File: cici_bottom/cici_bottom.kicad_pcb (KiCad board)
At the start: 2 copper layers, 88.4 x 132.8 mm, 8 parts

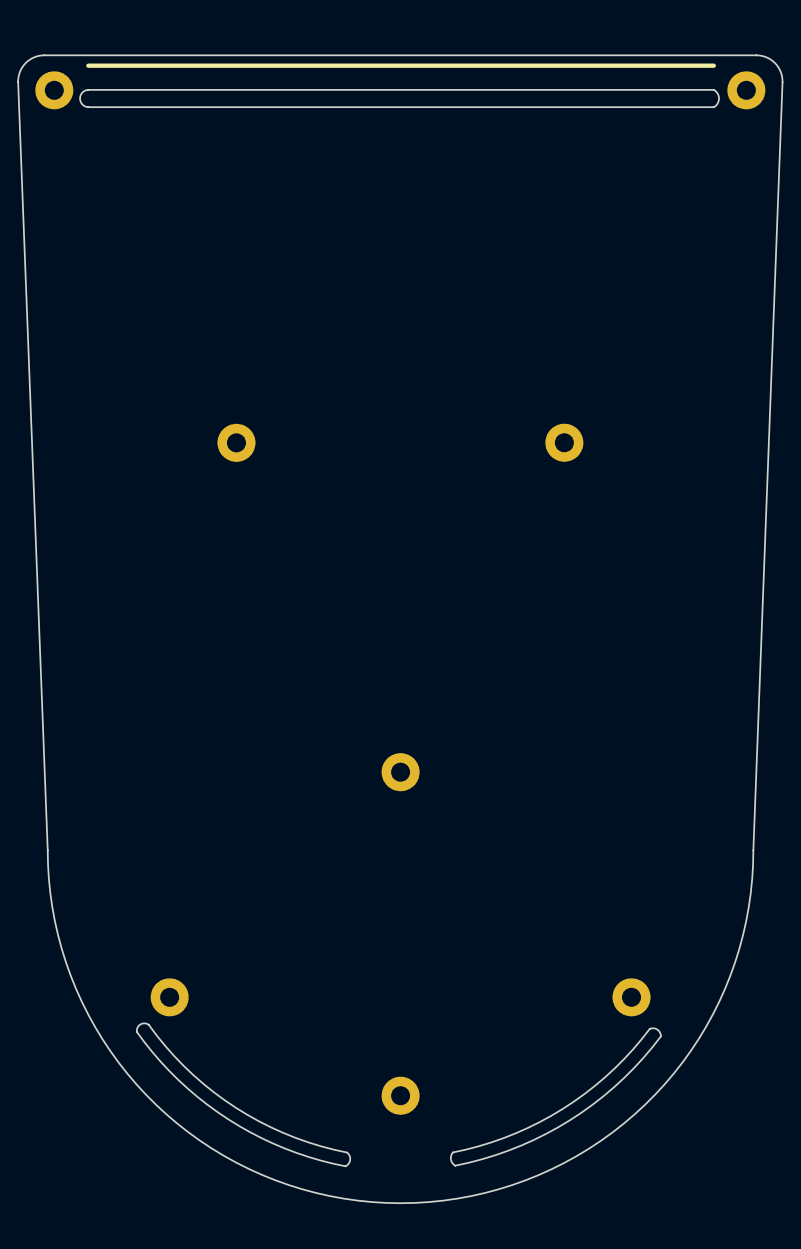
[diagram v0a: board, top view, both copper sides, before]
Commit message: prima versione conclusa. inizio seconda
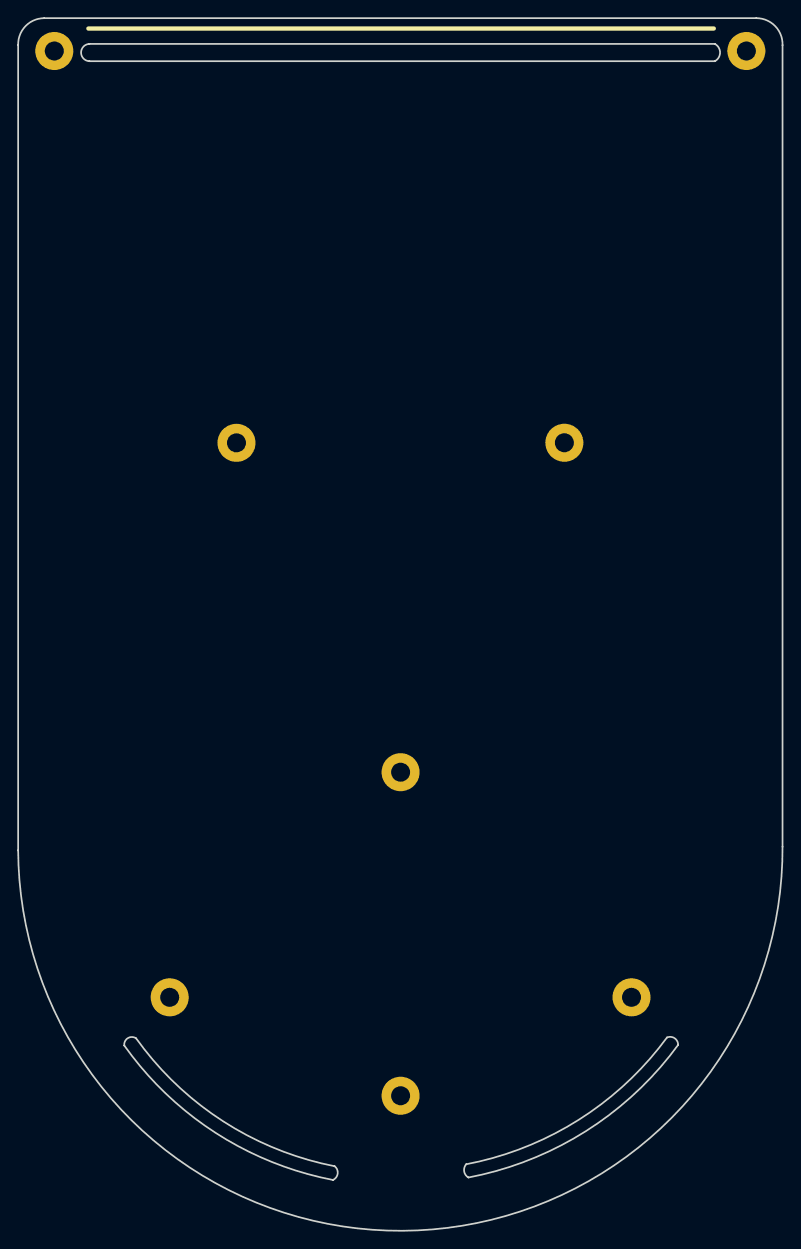
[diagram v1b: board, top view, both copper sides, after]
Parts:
- moved REF** 4.55 mm to (54.1, 25.5)
- moved REF** 4.55 mm to (134.1, 25.5)
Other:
- board size 88.4 x 132.8 mm -> 88.4 x 140.3 mm
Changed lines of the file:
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@@
   )
   (module MountingHole:MountingHole_2.2mm_M2_Pad (layer F.Cu)
-    (at 54.06 30.05)
+    (at 54.06 25.5)
     (descr "Mounting Hole 2.2mm, M2")
     (tags "mounting hole 2.2mm m2")
@@
   )
   (module MountingHole:MountingHole_2.2mm_M2_Pad (layer F.Cu)
-    (at 134.14 30.05)
+    (at 134.14 25.5)
     (descr "Mounting Hole 2.2mm, M2")
     (tags "mounting hole 2.2mm m2")
@@
     (pad 1 thru_hole circle (at 0 0) (size 4.4 4.4) (drill 2.2) (layers *.Cu *.Mask))
   )
-  (gr_line (start 58 27.2) (end 130.375 27.2) (layer F.SilkS) (width 0.5))
-  (gr_arc (start 123.33 139.5) (end 124.246762 139.525368) (angle -115.3397962) (layer Edge.Cuts) (width 0.2))
-  (gr_arc (start 100.95 153.61) (end 100.191271 152.951118) (angle -101.2542279) (layer Edge.Cuts) (width 0.2))
-  (gr_arc (start 64.48 138.89) (end 64.98 138.17) (angle -131.9838884) (layer Edge.Cuts) (width 0.2))
-  (gr_arc (start 87.37 153.7) (end 87.750789 154.553857) (angle -117.7344543) (layer Edge.Cuts) (width 0.2))
-  (gr_arc (start 92.926271 116.091118) (end 100.191271 152.951118) (angle -41.92680981) (layer Edge.Cuts) (width 0.2))
-  (gr_arc (start 95.075 116.675) (end 64.98 138.17) (angle -43.3547479) (layer Edge.Cuts) (width 0.2))
-  (gr_arc (start 92.925 116.1) (end 100.451863 154.482728) (angle -42.11246634) (layer Edge.Cuts) (width 0.2))
-  (gr_arc (start 95.075 116.675) (end 63.61 139) (angle -43.7) (layer Edge.Cuts) (width 0.2))
-  (gr_arc (start 58.04 31) (end 58 32) (angle 175.4) (layer Edge.Cuts) (width 0.2))
-  (gr_arc (start 129.84 31) (end 130.375 32) (angle -123.7064376) (layer Edge.Cuts) (width 0.2))
-  (gr_line (start 58 32) (end 130.375 32) (layer Edge.Cuts) (width 0.2))
-  (gr_line (start 58 30) (end 130.375 30) (layer Edge.Cuts) (width 0.2))
-  (gr_text CICI (at 94.125 153.3) (layer B.SilkS)
-    (effects (font (size 4 4) (thickness 0.5)) (justify mirror))
+  (gr_arc (start 85.92 155.28) (end 86.300789 156.133857) (angle -117.7344543) (layer Edge.Cuts) (width 0.2))
+  (gr_arc (start 63.03 140.47) (end 63.53 139.75) (angle -131.9838884) (layer Edge.Cuts) (width 0.2))
+  (gr_arc (start 93.625 118.255) (end 63.53 139.75) (angle -43.3547479) (layer Edge.Cuts) (width 0.2))
+  (gr_arc (start 93.625 118.255) (end 62.16 140.58) (angle -43.7) (layer Edge.Cuts) (width 0.2))
+  (gr_line (start 58 22.9) (end 130.375 22.9) (layer F.SilkS) (width 0.5))
+  (gr_arc (start 125.32217 140.491405) (end 126.238932 140.516773) (angle -115.3397962) (layer Edge.Cuts) (width 0.2))
+  (gr_arc (start 102.478137 154.977272) (end 101.719408 154.31839) (angle -101.2542279) (layer Edge.Cuts) (width 0.2))
+  (gr_arc (start 94.666271 117.411118) (end 101.719408 154.31839) (angle -42.88924805) (layer Edge.Cuts) (width 0.2))
+  (gr_arc (start 94.665 117.42) (end 101.98 155.85) (angle -43.03690352) (layer Edge.Cuts) (width 0.2))
+  (gr_arc (start 58.16 25.68) (end 58.12 26.68) (angle 175.4) (layer Edge.Cuts) (width 0.2))
+  (gr_arc (start 129.96 25.68) (end 130.495 26.68) (angle -123.7064376) (layer Edge.Cuts) (width 0.2))
+  (gr_line (start 58.12 26.68) (end 130.495 26.68) (layer Edge.Cuts) (width 0.2))
+  (gr_line (start 58.12 24.68) (end 130.495 24.68) (layer Edge.Cuts) (width 0.2))
+  (gr_text CICI (at 94.13 155.5) (layer B.SilkS)
+    (effects (font (size 3 4) (thickness 0.5)) (justify mirror))
   )
-  (gr_text -zanni- (at 94.125 149.7) (layer B.SilkS)
+  (gr_text -zanni- (at 94.13 152) (layer B.SilkS)
     (effects (font (size 1.5 1.5) (thickness 0.3)) (justify mirror))
   )
-  (gr_arc (start 92.925 116.1) (end 100.3 155.55) (angle -43.4) (layer B.SilkS) (width 0.5))
-  (gr_arc (start 95.075 116.675) (end 62.9 139.75) (angle -44.1) (layer B.SilkS) (width 0.5))
-  (gr_arc (start 94.15 117.85) (end 54.525 118.4) (angle -179.2) (layer B.SilkS) (width 0.5))
-  (gr_line (start 54.525 118.4) (end 51.100929 34) (layer B.SilkS) (width 0.5))
-  (gr_line (start 137.153817 34) (end 133.778817 117.853305) (layer B.SilkS) (width 0.5))
-  (gr_line (start 58 27.2) (end 130.375 27.2) (layer B.SilkS) (width 0.5))
-  (gr_arc (start 135.3 29.025) (end 138.325 29.125) (angle -91.9) (layer Edge.Cuts) (width 0.2))
-  (gr_line (start 138.325 29.125) (end 134.95 118) (layer Edge.Cuts) (width 0.2))
-  (gr_arc (start 94.125 118) (end 53.3 118) (angle -180) (layer Edge.Cuts) (width 0.2))
-  (gr_line (start 53.3 118) (end 49.875929 29.099977) (layer Edge.Cuts) (width 0.2))
-  (gr_arc (start 52.9 29.025) (end 52.9 26) (angle -91.4) (layer Edge.Cuts) (width 0.2))
-  (gr_line (start 52.9 26) (end 135.3 26) (layer Edge.Cuts) (width 0.2))
+  (gr_arc (start 94.1227 117.42) (end 100.53 158.33) (angle -43.4) (layer B.SilkS) (width 0.5))
+  (gr_arc (start 94.1227 117.42) (end 61.73 143.22) (angle -42.90512361) (layer B.SilkS) (width 0.5))
+  (gr_arc (start 94.1227 117.42) (end 51.100929 118.4) (angle -179.2) (layer B.SilkS) (width 0.5))
+  (gr_line (start 51.100929 118.4) (end 51.100929 30) (layer B.SilkS) (width 0.5))
+  (gr_line (start 137.153817 30) (end 137.153382 117.859999) (layer B.SilkS) (width 0.5))
+  (gr_line (start 58 22.9) (end 130.375 22.9) (layer B.SilkS) (width 0.5))
+  (gr_arc (start 135.3 24.725) (end 138.325 24.825) (angle -91.9) (layer Edge.Cuts) (width 0.2))
+  (gr_line (start 138.325 24.825) (end 138.324097 117.58) (layer Edge.Cuts) (width 0.2))
+  (gr_arc (start 94.1 117.79) (end 49.875903 118) (angle -180) (layer Edge.Cuts) (width 0.2))
+  (gr_line (start 49.875903 118) (end 49.875903 24.798907) (layer Edge.Cuts) (width 0.2))
+  (gr_arc (start 52.9 24.725) (end 52.9 21.7) (angle -91.4) (layer Edge.Cuts) (width 0.2))
+  (gr_line (start 52.9 21.7) (end 135.299651 21.698348) (layer Edge.Cuts) (width 0.2))
 )
